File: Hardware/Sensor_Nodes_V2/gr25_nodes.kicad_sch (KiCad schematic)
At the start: 48 parts, among them J1 SWD, J2 IO1, J3 I02, J4 PWR, U1 SN65HVD230, U2 AP63205WU, U3 AMS1117-3.3, U4 STM32F103C8Tx, Y1 16MHz

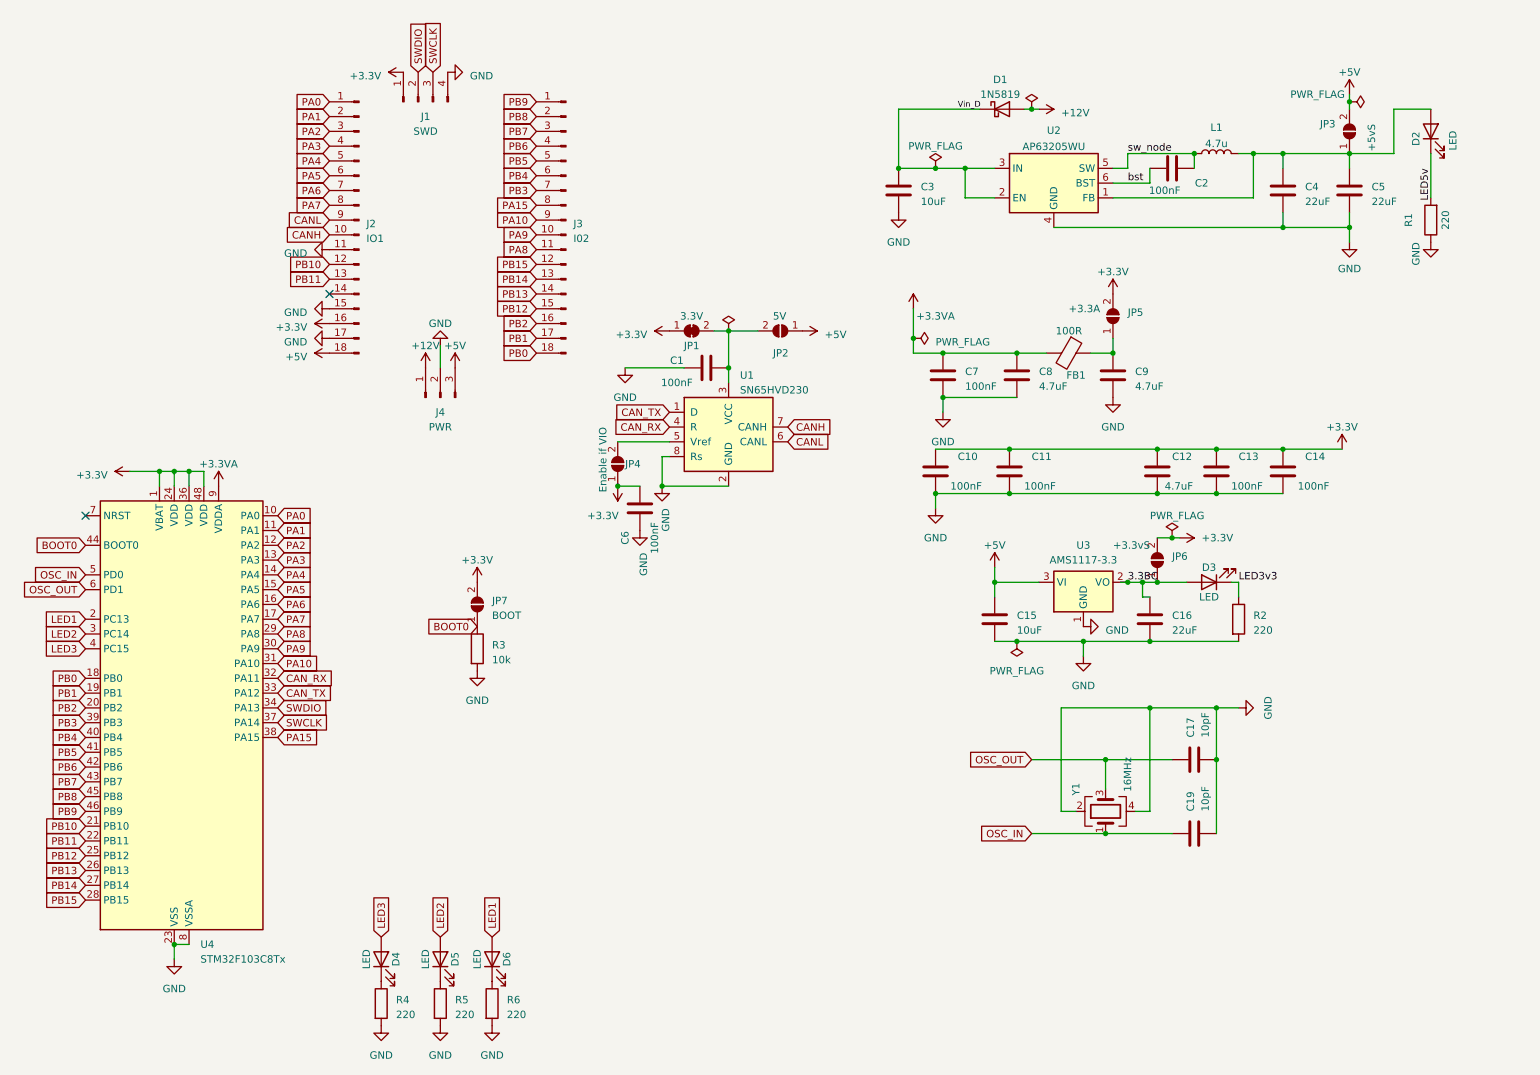
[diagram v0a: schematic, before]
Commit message: some chnages, for tracking purpose
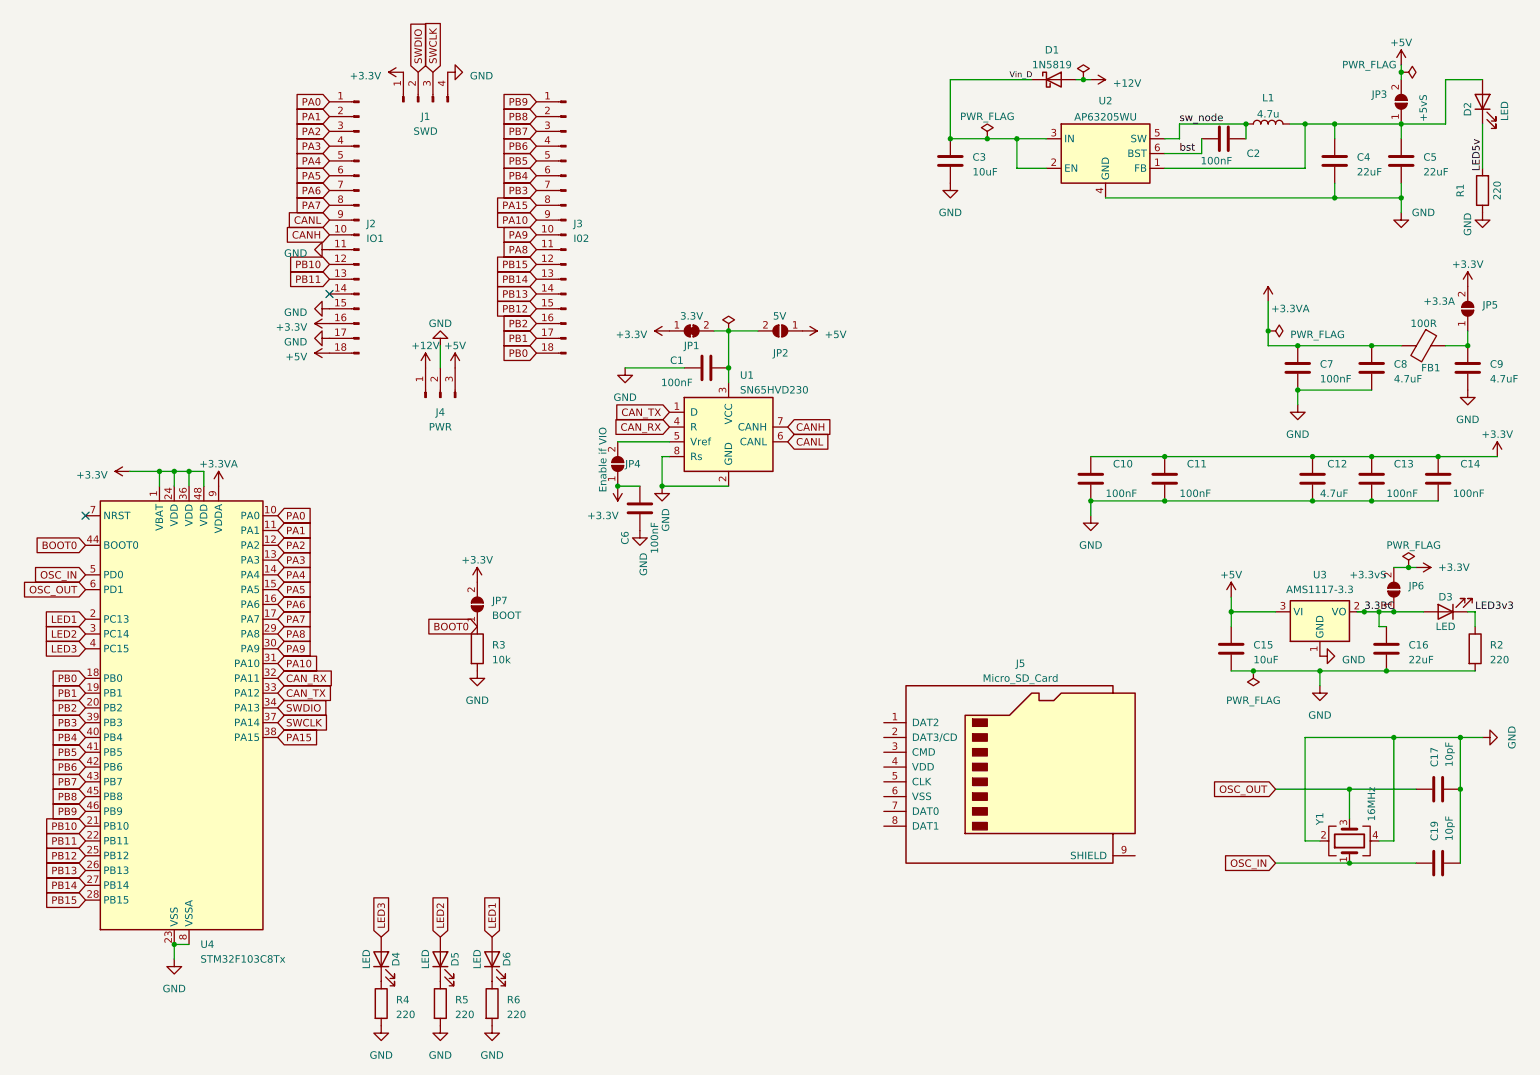
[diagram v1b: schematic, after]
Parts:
- added J5: Micro_SD_Card, symbol Connector:Micro_SD_Card
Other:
- moved on the sheet: C10, C11, C12, C13, C14, C15, C16, C17, C19, C2, C3, C4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
